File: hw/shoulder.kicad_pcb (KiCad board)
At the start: 2 copper layers, 60 x 40 mm, 27 parts, among them J1 IDC_02X07, U1 OSRB38C9BA, U2 OSRB38C9BA, U3 OSRB38C9BA, U4 OSRB38C9BA, U5 OSRB38C9BA

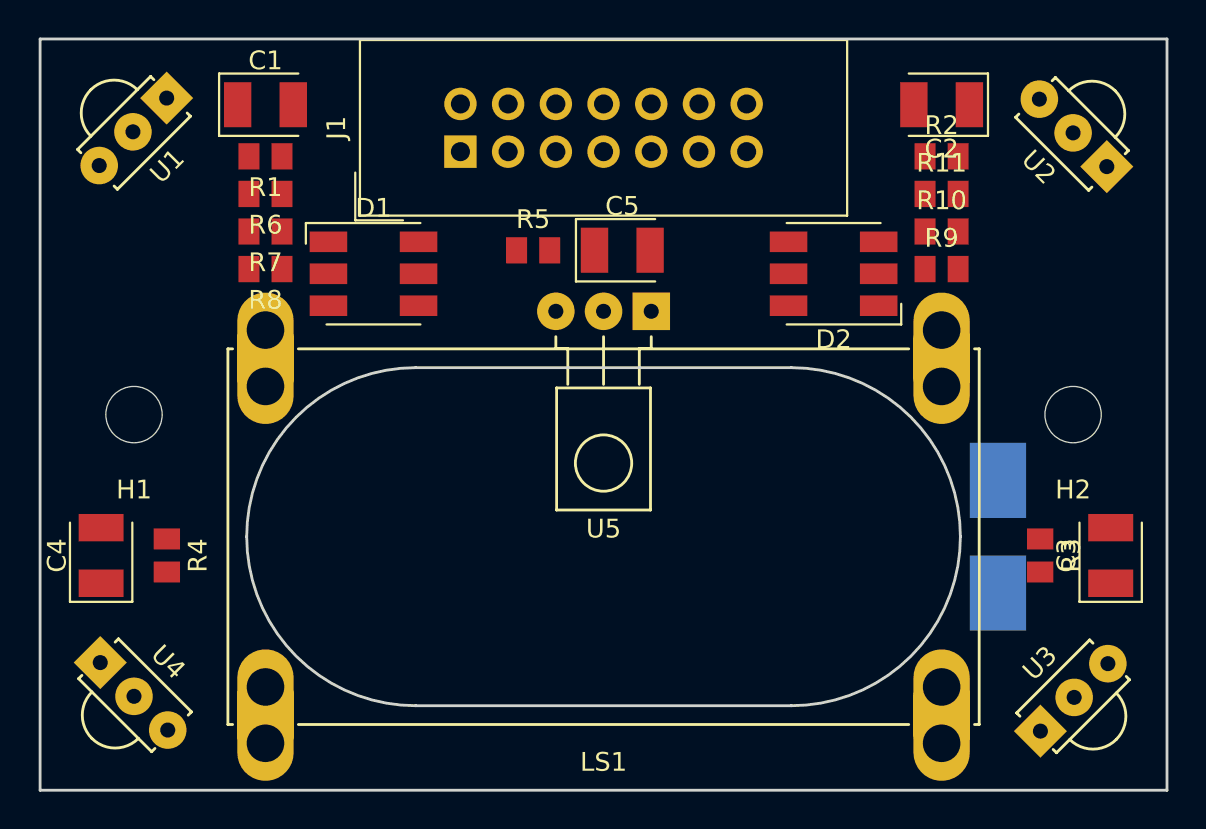
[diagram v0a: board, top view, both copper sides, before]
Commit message: updated pcb
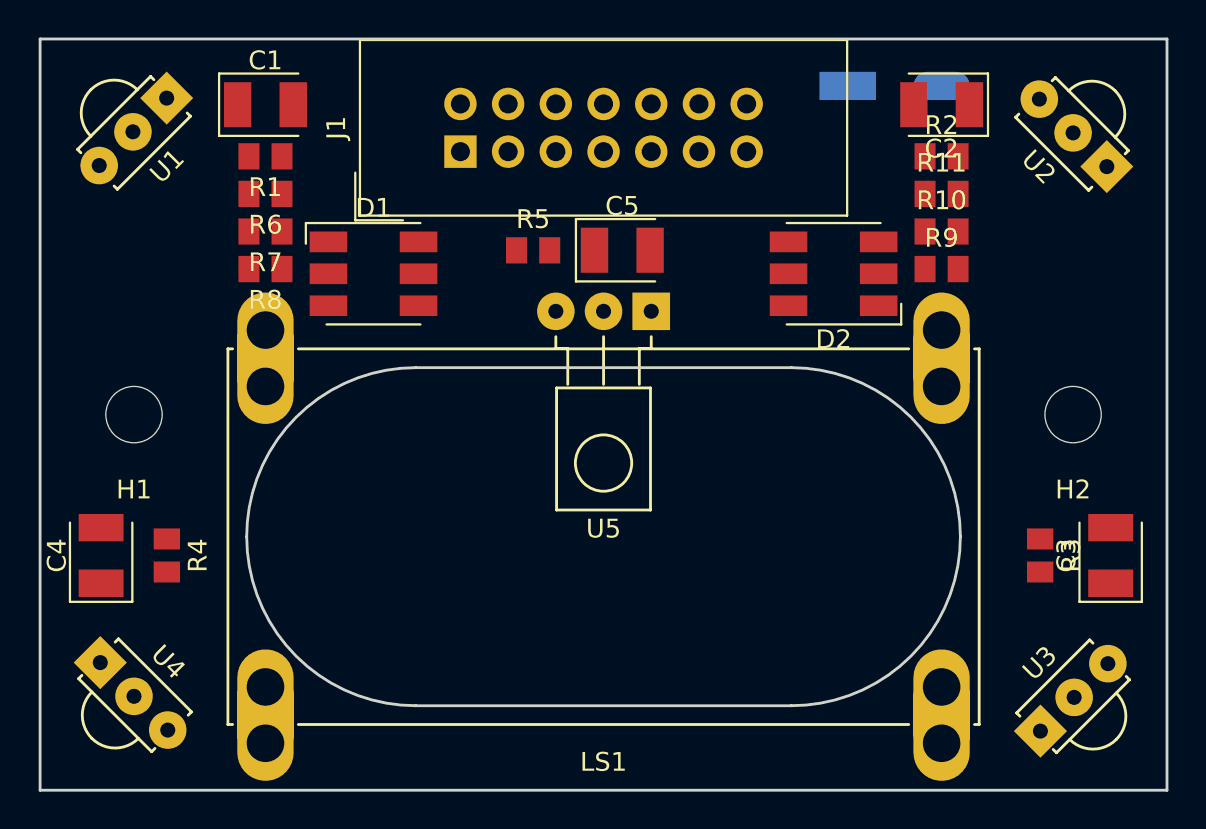
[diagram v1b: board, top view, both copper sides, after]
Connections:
- LS1 pad 3: Net-(LS1-Pad3) -> GND
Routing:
- added copper zone on B.Cu, net GND
- added copper zone on F.Cu, net GND
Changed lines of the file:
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@@
     (zones 0)
     (modules 27)
-    (nets 21)
+    (nets 20)
   )
   (page A4)
@@
   (setup
     (last_trace_width 0.25)
+    (user_trace_width 0.5)
+    (user_trace_width 1)
     (trace_clearance 0.2)
     (zone_clearance 0.508)
@@
     (mod_text_size 1 1)
     (mod_text_width 0.15)
-    (pad_size 1.524 1.524)
-    (pad_drill 0.762)
+    (pad_size 6 3)
+    (pad_drill 2)
     (pad_to_mask_clearance 0.2)
     (aux_axis_origin 0 0)
@@
   (net 18 /SP+)
   (net 19 /SP-)
-  (net 20 "Net-(LS1-Pad3)")
   (net_class Default "Toto je výchozí třída sítě."
     (clearance 0.2)
@@
     (add_net "Net-(D2-Pad2)")
     (add_net "Net-(D2-Pad3)")
-    (add_net "Net-(LS1-Pad3)")
   )
   (module KLIB_Audio:REP-ABS-224-RC (layer F.Cu)
@@
     (fp_line (start 10 -20) (end 10 -19.75) (layer F.SilkS) (width 0.15))
     (fp_line (start -10 -20) (end -10 -19.75) (layer F.SilkS) (width 0.15))
-    (pad 1 smd rect (at -3 21 90) (size 4 3) (layers B.Cu B.Paste B.Mask)
+    (pad 1 smd rect (at 24 13 90) (size 1.5 3) (layers B.Cu B.Paste B.Mask)
       (net 18 /SP+))
-    (pad 2 smd rect (at 3 21 90) (size 4 3) (layers B.Cu B.Paste B.Mask)
+    (pad 2 smd oval (at 24 18 90) (size 1.5 3) (layers B.Cu B.Paste B.Mask)
       (net 19 /SP-))
     (pad 3 thru_hole oval (at 8 18 90) (size 6 3) (drill 2 (offset 1 0)) (layers *.Cu *.Mask)
-      (net 20 "Net-(LS1-Pad3)"))
+      (net 17 GND) (zone_connect 2))
     (pad 3 thru_hole oval (at 8 -18 90) (size 6 3) (drill 2 (offset 1 0)) (layers *.Cu *.Mask)
-      (net 20 "Net-(LS1-Pad3)"))
+      (net 17 GND) (zone_connect 2))
     (pad 3 thru_hole oval (at -8 -18 90) (size 6 3) (drill 2 (offset -1 0)) (layers *.Cu *.Mask)
-      (net 20 "Net-(LS1-Pad3)"))
+      (net 17 GND) (zone_connect 2))
     (pad 3 thru_hole oval (at -8 18 90) (size 6 3) (drill 2 (offset -1 0)) (layers *.Cu *.Mask)
-      (net 20 "Net-(LS1-Pad3)"))
+      (net 17 GND) (zone_connect 2))
     (pad 3 thru_hole oval (at 11 -18 90) (size 6 3) (drill 2 (offset -1 0)) (layers *.Cu *.Mask)
-      (net 20 "Net-(LS1-Pad3)"))
+      (net 17 GND) (zone_connect 2))
     (pad 3 thru_hole oval (at -11 -18 90) (size 6 3) (drill 2 (offset 1 0)) (layers *.Cu *.Mask)
-      (net 20 "Net-(LS1-Pad3)"))
+      (net 17 GND) (zone_connect 2))
     (pad 3 thru_hole oval (at 11 18 90) (size 6 3) (drill 2 (offset -1 0)) (layers *.Cu *.Mask)
-      (net 20 "Net-(LS1-Pad3)"))
+      (net 17 GND) (zone_connect 2))
     (pad 3 thru_hole oval (at -11 18 90) (size 6 3) (drill 2 (offset 1 0)) (layers *.Cu *.Mask)
-      (net 20 "Net-(LS1-Pad3)"))
+      (net 17 GND) (zone_connect 2))
     (model "$(KIPRJMOD)/project.3dshapes/ABS-224-RC.wrl"
       (at (xyz 0 0 0))
@@
   (gr_line (start 185 120) (end 185 80) (layer Edge.Cuts) (width 0.15))
   (gr_line (start 125 120) (end 185 120) (layer Edge.Cuts) (width 0.15))
+  (zone (net 17) (net_name GND) (layer F.Cu) (hatch edge 0.508)
+    (connect_pads (clearance 0.508))
+    (min_thickness 0.254)
+    (fill yes (arc_segments 16) (thermal_gap 0.508) (thermal_bridge_width 0.508))
+    (polygon
+      (pts
+        (xy 125 120) (xy 185 120) (xy 185 80) (xy 125 80)
+      )
+    )
+  )
+  (zone (net 17) (net_name GND) (layer B.Cu) (hatch edge 0.508)
+    (connect_pads (clearance 0.508))
+    (min_thickness 0.254)
+    (fill yes (arc_segments 16) (thermal_gap 0.508) (thermal_bridge_width 0.508))
+    (polygon
+      (pts
+        (xy 125 80) (xy 185 80) (xy 185 120) (xy 125 120)
+      )
+    )
+  )
 )
